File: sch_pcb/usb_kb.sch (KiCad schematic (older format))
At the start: 12 parts, among them P1 USB_C_Plug, U1 STM32F103C6Tx, U2 AMS1117-3.3, U3 AMS1117-3.3

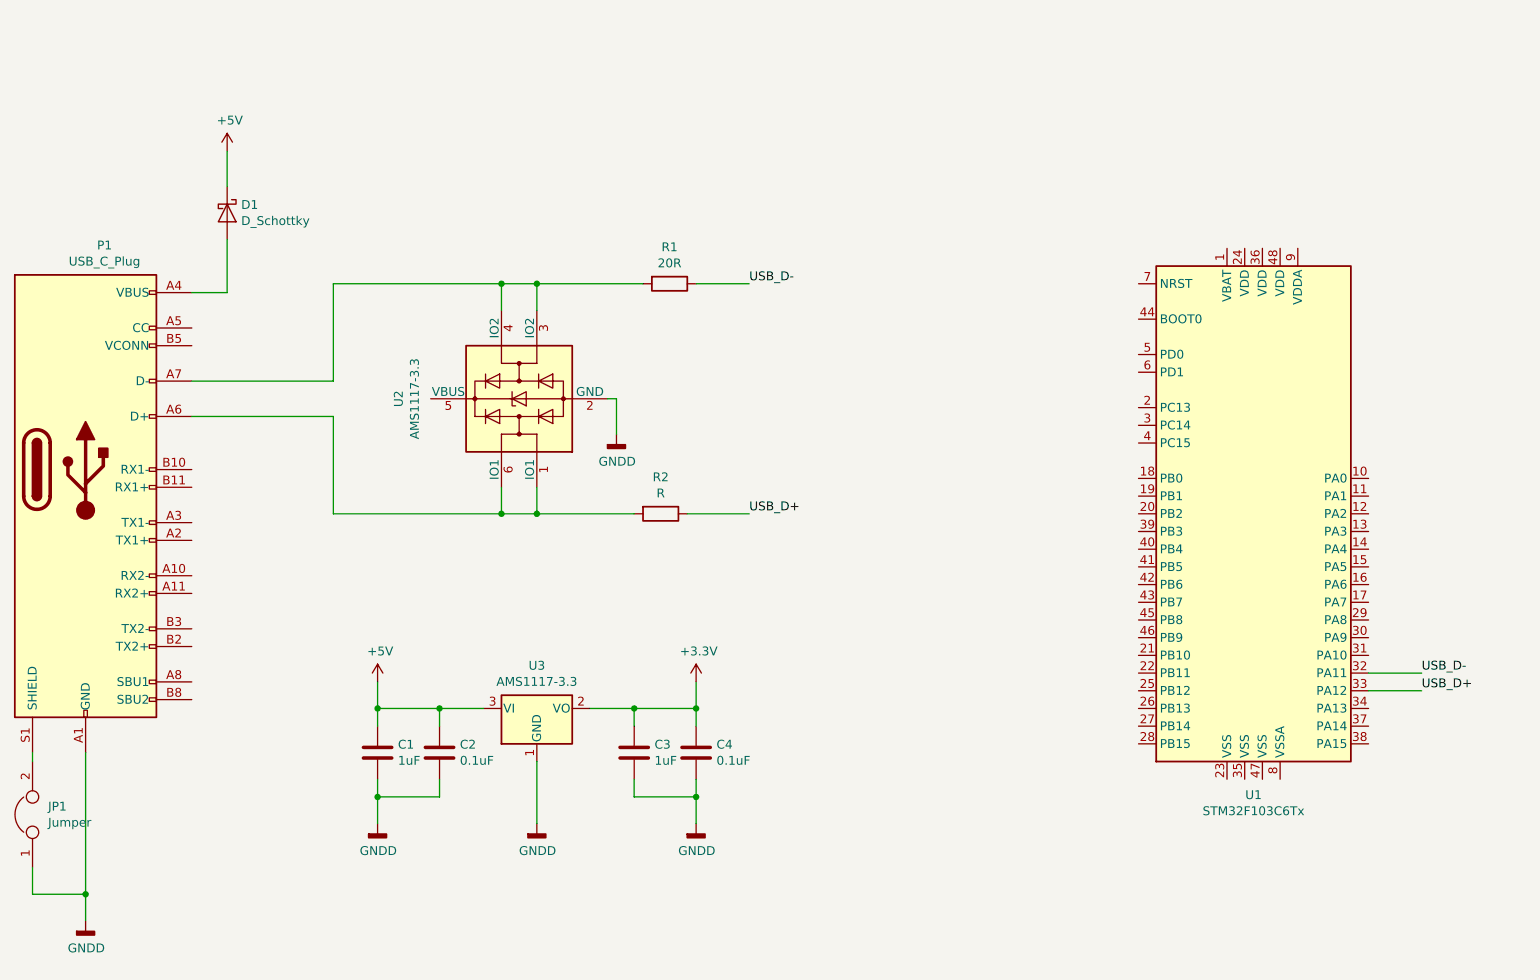
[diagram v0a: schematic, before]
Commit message: Андрей добавил питание, Никита доделал
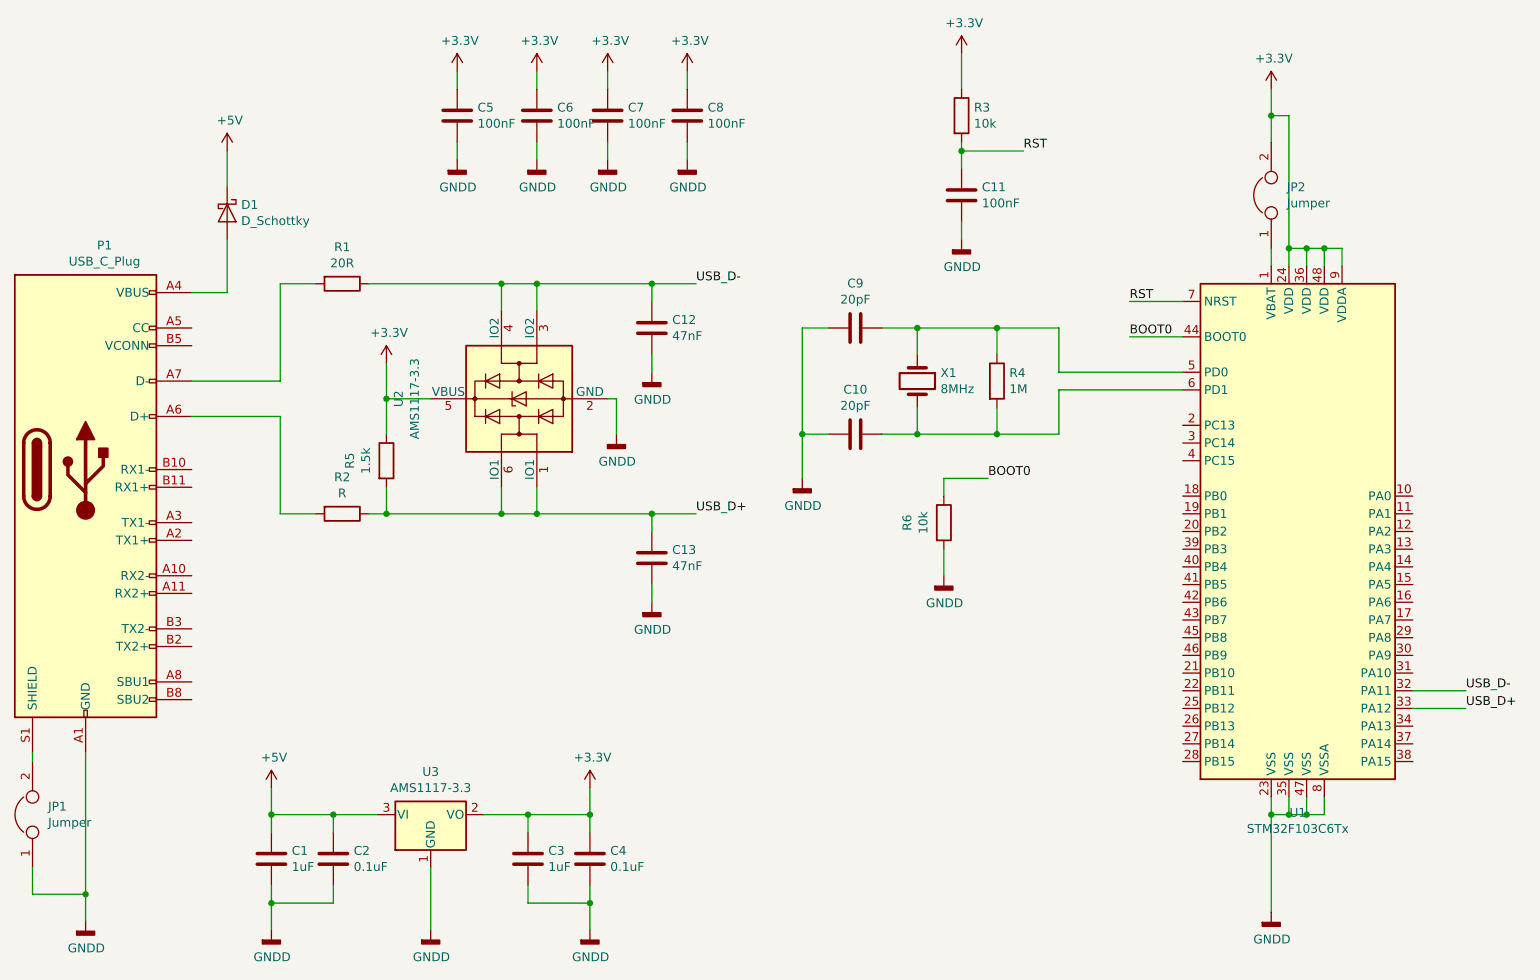
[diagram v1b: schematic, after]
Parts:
- added C10, C9: 20pF, Capacitor_SMD:C_0805_2012Metric_Pad1.15x1.40mm_HandSolder, symbol Device:C
- added C11, C5, C6, C7, C8: 100nF, Capacitor_SMD:C_0805_2012Metric_Pad1.15x1.40mm_HandSolder, symbol Device:C
- added C12, C13: 47nF, Capacitor_SMD:C_0805_2012Metric_Pad1.15x1.40mm_HandSolder, symbol Device:C
- added JP2: Jumper, Jumper:SolderJumper-2_P1.3mm_Open_TrianglePad1.0x1.5mm, symbol Device:Jumper
- added R3, R6: 10k, Resistor_SMD:R_0603_1608Metric_Pad1.05x0.95mm_HandSolder, symbol Device:R
- added R4: 1M, Resistor_SMD:R_0603_1608Metric_Pad1.05x0.95mm_HandSolder, symbol Device:R
- added R5: 1.5k, Resistor_SMD:R_0603_1608Metric_Pad1.05x0.95mm_HandSolder, symbol Device:R
- added X1: 8MHz, Crystal:Crystal_HC49-4H_Vertical, symbol Device:Crystal
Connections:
- net +3V3: now also U1.24 (VDD), U1.36 (VDD), U1.48 (VDD), U1.9 (VDDA), U2.5 (VBUS), C5.1, C6.1, C7.1, C8.1, JP2.2, R3.1, R5.1
- net GNDD: now also U1.23 (VSS), U1.35 (VSS), U1.47 (VSS), U1.8 (VSSA), C10.2, C11.2, C12.2, C13.2, C5.2, C6.2, C7.2, C8.2, C9.2, R6.2
- net USB_D+: now also U2.1 (IO1), U2.6 (IO1), C13.1, R5.2
- net USB_D-: now also U2.3 (IO2), U2.4 (IO2), C12.1
- net at P1.A6 (D+), R2.2: no longer U2.1 (IO1), U2.6 (IO1)
- net at P1.A7 (D-), R1.2: no longer U2.3 (IO2), U2.4 (IO2)
- net at U1.1 (VBAT): now also JP2.1
- net BOOT0: now reaches U1.44 (BOOT0)
- net BOOT0: now also R6.1
- net at U1.5 (PD0): now also C9.1, R4.1, X1.1
- net at U1.6 (PD1): now also C10.1, R4.2, X1.2
- net RST: now reaches U1.7 (NRST)
- net RST: now also C11.1, R3.2
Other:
- moved on the sheet: C1, C2, C3, C4, R1, R2, U1, U3
